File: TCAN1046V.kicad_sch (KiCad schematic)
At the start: 5 parts, among them U2 TCAN1051VDRBRQ1

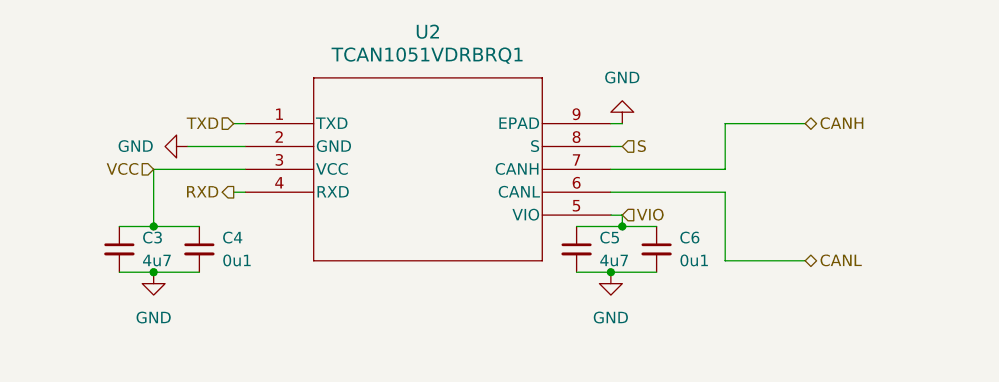
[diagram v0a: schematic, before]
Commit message: OBC: Continue PCB lauout
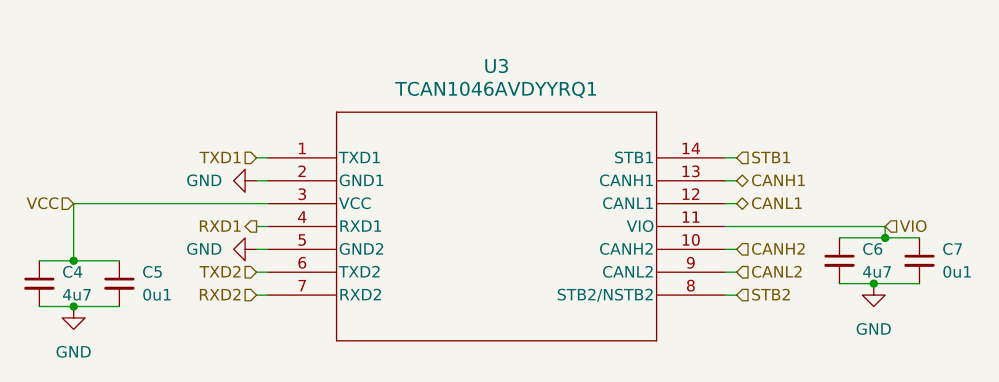
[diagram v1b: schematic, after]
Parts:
- removed U2: TCAN1051VDRBRQ1, TCAN1051V:DRB8_TEX, symbol TCAN1051V:TCAN1051VDRBRQ1
- added U3: TCAN1046AVDYYRQ1, TCAN1046AV:SOT23_DYY_TEX, symbol TCAN1046AVDYYRQ1:TCAN1046AVDYYRQ1
- renumbered C3 to C4, C4 to C5, C5 to C6, C6 to C7
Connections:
- net GND: now also U3.2 (GND1), U3.5 (GND2)
- net VCC: now also U3.3 (VCC)
- net VIO: now also U3.11 (VIO)
- new net CANH1: U3.13 (CANH1)
- new net CANH2: U3.10 (CANH2)
- new net CANL1: U3.12 (CANL1)
- new net CANL2: U3.9 (CANL2)
- new net RXD1: U3.4 (RXD1)
- new net RXD2: U3.7 (RXD2)
- new net STB1: U3.14 (STB1)
- new net STB2: U3.8 (STB2/NSTB2)
- new net TXD1: U3.1 (TXD1)
- new net TXD2: U3.6 (TXD2)
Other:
- moved on the sheet: C4, C5, C6, C7
